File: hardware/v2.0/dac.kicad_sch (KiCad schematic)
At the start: 1 part, among them IC3 LTC2630ISC6-LZ12#TRMPBF

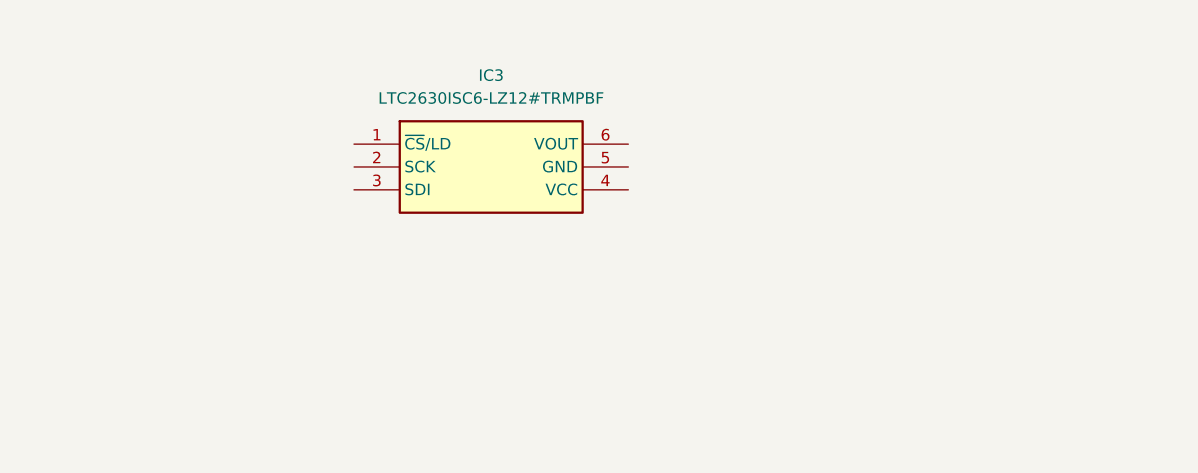
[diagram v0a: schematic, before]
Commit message: DAC Vout
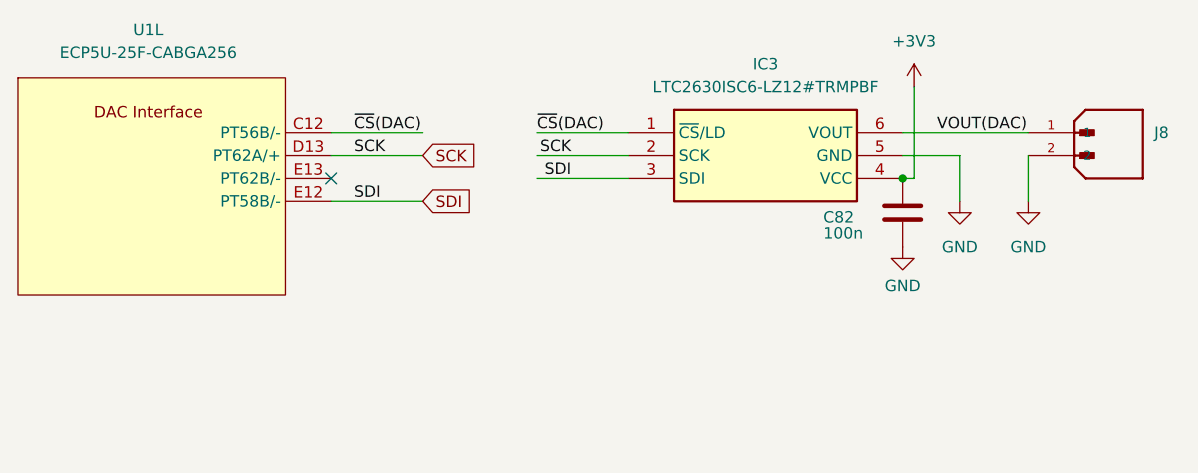
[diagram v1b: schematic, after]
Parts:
- added C82: 100n, Capacitor_SMD:C_0402_1005Metric, symbol Device:C
- added J8: 530480210, 530480210:MOLEX_530480210, symbol 530480210:530480210
- added U1: ECP5U-25F-CABGA256, Package_BGA:BGA-256_14.0x14.0mm_Layout16x16_P0.8mm_Ball0.45mm_Pad0.32mm_NSMD, symbol icepi-lib:LFE5U-25F-6BG256x
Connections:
- net ~{CS}(DAC): now reaches IC3.1 (~{CS}/LD)
- net ~{CS}(DAC): now also U1.C12 (PT56B/-)
- net SCK: now reaches IC3.2 (SCK)
- net SCK: now also U1.D13 (PT62A/+)
- net SDI: now reaches IC3.3 (SDI)
- net SDI: now also U1.E12 (PT58B/-)
- net +3V3: now reaches IC3.4 (VCC)
- net +3V3: now also C82.1
- net GND: now reaches IC3.5 (GND)
- net GND: now also C82.2, J8.2
- net VOUT(DAC): now reaches IC3.6 (VOUT)
- net VOUT(DAC): now also J8.1
- no-connect marks 0 -> 1
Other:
- moved on the sheet: IC3
